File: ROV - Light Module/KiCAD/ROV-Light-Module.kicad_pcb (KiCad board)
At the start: 2 copper layers, 73.7 x 23.4 mm, 53 parts, among them J1 AVR UPDI Header, J4 Conn_02x05_Odd_Even, J6 Main In, J7 Conn_02x05_Odd_Even, J8 Middle - Top, J9 Middle - Top, U1 AL8805W5, U2 ATtiny1614-Arduino, U3 AP63205WU, U6 MAX13487E

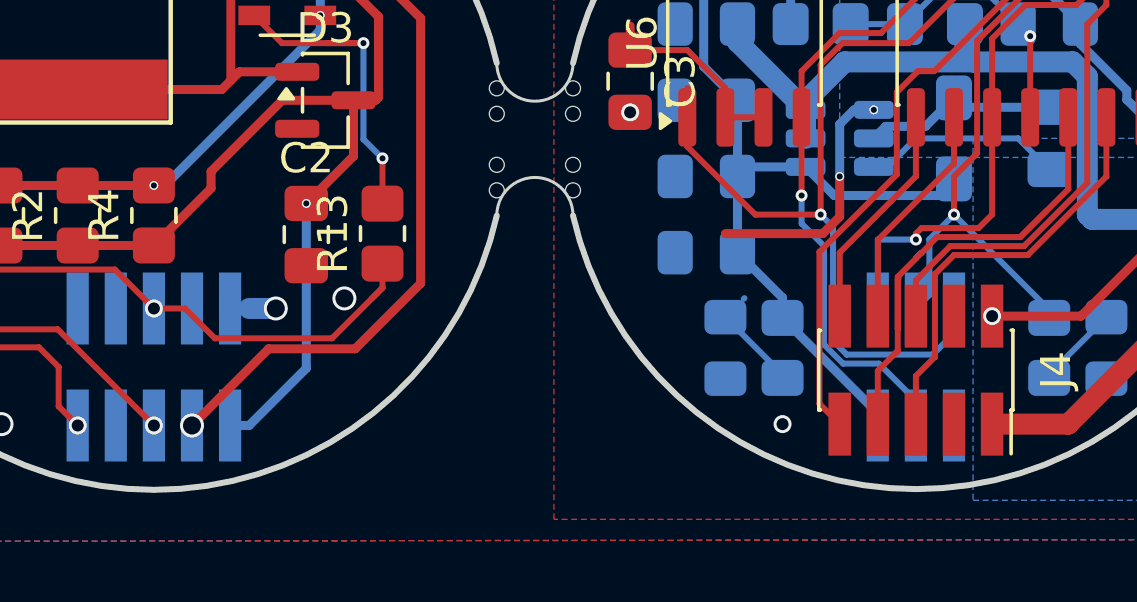
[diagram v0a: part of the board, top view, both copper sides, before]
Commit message: massive cleanup
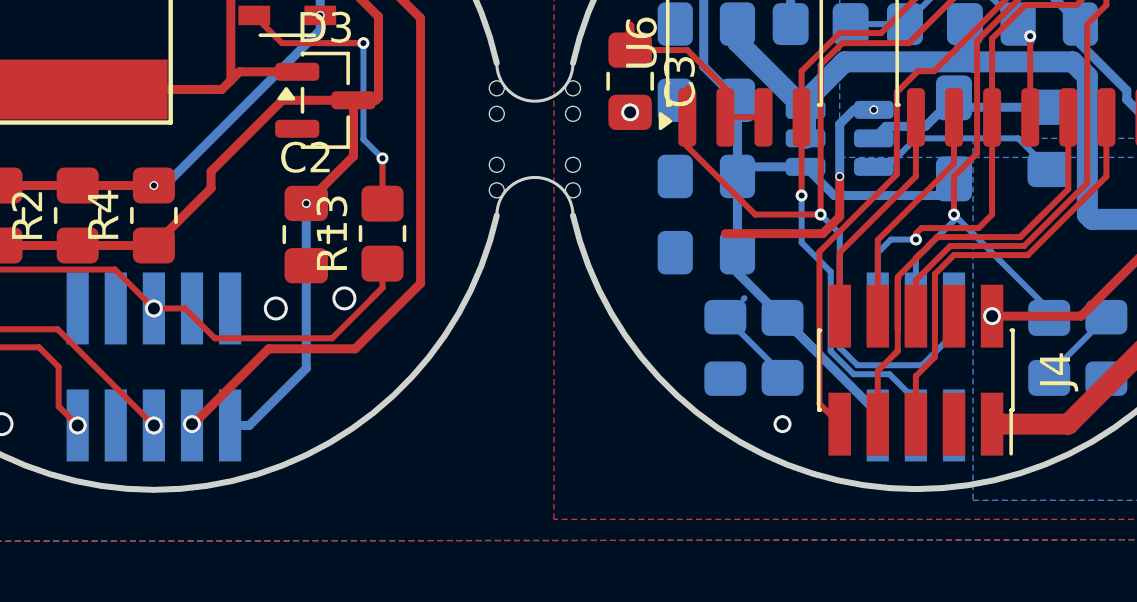
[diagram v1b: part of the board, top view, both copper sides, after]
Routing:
- net +5V: track 34.8 -> 36.4 mm
- net GND: track 54.1 -> 53.2 mm
- net /Arduino Driver PCB/Builtin_LED: track 18.6 -> 17.8 mm
